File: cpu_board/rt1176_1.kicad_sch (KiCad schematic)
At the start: 46 parts, among them SW1 SWITCH_SMT4.6X2.8, U2 MIMXRT1176

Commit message: add models and power diagram
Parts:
- U2, U? (x4): footprint adcs:BGA289C80P17X17_1400X14000X152 -> adcs:U_MIMXRT1176DVMAA_NXP
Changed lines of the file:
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@@
       (effects (font (size 1.27 1.27)))
     )
-    (property "Footprint" "adcs:BGA289C80P17X17_1400X14000X152" (at 223.52 67.31 0)
+    (property "Footprint" "adcs:U_MIMXRT1176DVMAA_NXP" (at 223.52 67.31 0)
       (effects (font (size 1.27 1.27)) hide)
     )
@@
       (effects (font (size 1.27 1.27)) hide)
     )
+    (property "DigiKey Part Number" "" (at 223.52 66.04 0)
+      (effects (font (size 1.27 1.27)) hide)
+    )
+    (property "Tolerance" "" (at 223.52 66.04 0)
+      (effects (font (size 1.27 1.27)))
+    )
+    (property "Power Rating" "" (at 223.52 66.04 0)
+      (effects (font (size 1.27 1.27)))
+    )
     (pin "L9")
     (pin "M10")
@@
       (effects (font (size 1.27 1.27)))
     )
-    (property "Footprint" "adcs:BGA289C80P17X17_1400X14000X152" (at 220.98 142.24 0)
+    (property "Footprint" "adcs:U_MIMXRT1176DVMAA_NXP" (at 220.98 142.24 0)
       (effects (font (size 1.27 1.27)) hide)
     )
@@
       (effects (font (size 1.27 1.27)) hide)
     )
+    (property "DigiKey Part Number" "" (at 220.98 140.97 0)
+      (effects (font (size 1.27 1.27)) hide)
+    )
+    (property "Tolerance" "" (at 220.98 140.97 0)
+      (effects (font (size 1.27 1.27)))
+    )
+    (property "Power Rating" "" (at 220.98 140.97 0)
+      (effects (font (size 1.27 1.27)))
+    )
     (pin "L9")
     (pin "M10")
@@
       (effects (font (size 1.27 1.27)))
     )
-    (property "Footprint" "adcs:BGA289C80P17X17_1400X14000X152" (at 50.8 240.03 0)
+    (property "Footprint" "adcs:U_MIMXRT1176DVMAA_NXP" (at 50.8 240.03 0)
       (effects (font (size 1.27 1.27)) hide)
     )
@@
       (effects (font (size 1.27 1.27)) hide)
     )
+    (property "DigiKey Part Number" "" (at 50.8 238.76 0)
+      (effects (font (size 1.27 1.27)) hide)
+    )
+    (property "Tolerance" "" (at 50.8 238.76 0)
+      (effects (font (size 1.27 1.27)))
+    )
+    (property "Power Rating" "" (at 50.8 238.76 0)
+      (effects (font (size 1.27 1.27)))
+    )
     (pin "L9")
     (pin "M10")
@@
       (effects (font (size 1.27 1.27)))
     )
-    (property "Footprint" "adcs:BGA289C80P17X17_1400X14000X152" (at 220.98 200.66 0)
+    (property "Footprint" "adcs:U_MIMXRT1176DVMAA_NXP" (at 220.98 200.66 0)
       (effects (font (size 1.27 1.27)) hide)
     )
@@
       (effects (font (size 1.27 1.27)) hide)
     )
+    (property "DigiKey Part Number" "" (at 220.98 199.39 0)
+      (effects (font (size 1.27 1.27)) hide)
+    )
+    (property "Tolerance" "" (at 220.98 199.39 0)
+      (effects (font (size 1.27 1.27)))
+    )
+    (property "Power Rating" "" (at 220.98 199.39 0)
+      (effects (font (size 1.27 1.27)))
+    )
     (pin "L9")
     (pin "M10")
@@
       (effects (font (size 1.27 1.27)))
     )
-    (property "Footprint" "adcs:BGA289C80P17X17_1400X14000X152" (at 219.71 255.27 0)
+    (property "Footprint" "adcs:U_MIMXRT1176DVMAA_NXP" (at 219.71 255.27 0)
       (effects (font (size 1.27 1.27)) hide)
     )
@@
       (effects (font (size 1.27 1.27)) hide)
     )
+    (property "DigiKey Part Number" "" (at 219.71 254 0)
+      (effects (font (size 1.27 1.27)) hide)
+    )
+    (property "Tolerance" "" (at 219.71 254 0)
+      (effects (font (size 1.27 1.27)))
+    )
+    (property "Power Rating" "" (at 219.71 254 0)
+      (effects (font (size 1.27 1.27)))
+    )
     (pin "L9")

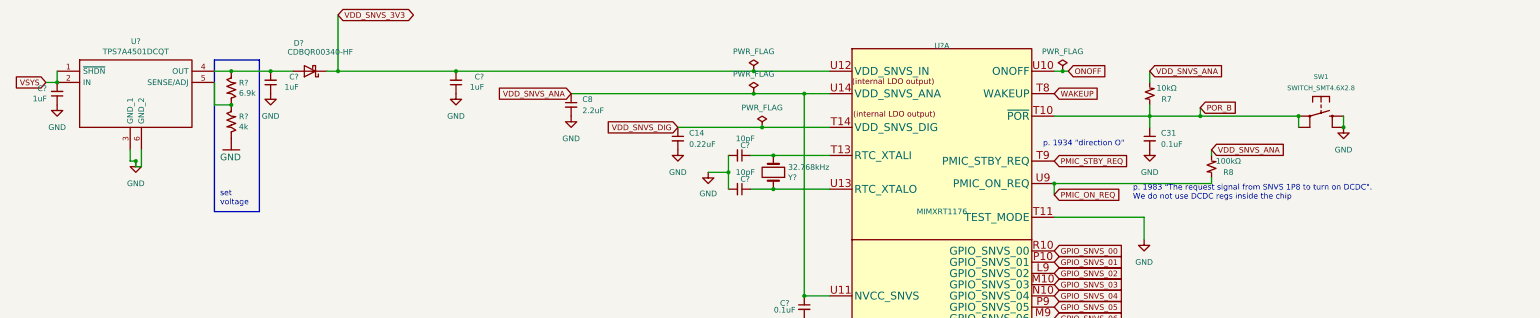
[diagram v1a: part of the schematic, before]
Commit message: continue work on fanout
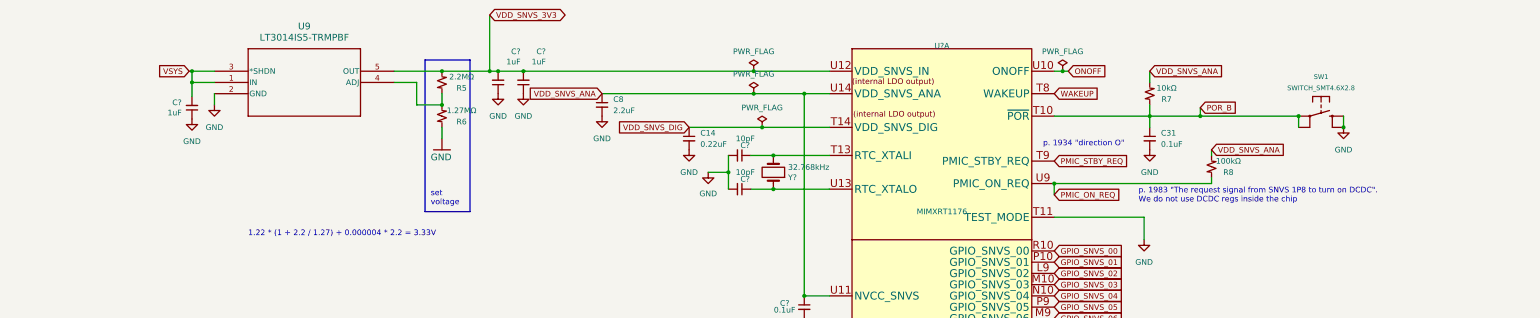
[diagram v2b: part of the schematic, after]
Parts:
- removed C?: 1uF, Capacitor_SMD:C_0402_1005Metric, symbol Device:C_Small
- removed D?: CDBQR00340-HF, adcs:D0402_H0.55MM, symbol Device:D_Schottky
- removed R?: 4k, Resistor_SMD:R_0402_1005Metric, symbol Device:R_US
- removed R?: 6.9k, Resistor_SMD:R_0402_1005Metric, symbol Device:R_US
- removed U?: TPS7A4501DCQT, mainboard:TPS7A4501DCQT, symbol mainboard:TPS7A4501DCQT
- added C?: 1uF, adcs:Perfect_0201, symbol Device:C_Small
- added R5: 2.2MΩ, adcs:Perfect_0402, symbol Device:R_Small_US
- added R6: 1.27MΩ, adcs:Perfect_0402, symbol Device:R_Small_US
- added U9: LT3014IS5-TRMPBF, adcs:S_5_ADI, symbol adcs:LT3014IS5-TRMPBF
- C10, C12, C13, C14, C15, C23, C26, C31, C34, C38, C40, C41, C42, C43, C8, C? (x3): footprint Capacitor_SMD:C_0402_1005Metric -> adcs:Perfect_0201
- C17, C22, C9: footprint Capacitor_SMD:C_0402_1005Metric -> adcs:Perfect_0201; Footprint (for JLCPCB) 0402 -> 0201
- C4, C? (x4): footprint Capacitor_SMD:C_0402_1005Metric -> adcs:Perfect_0402
- C6: footprint Capacitor_SMD:C_0402_1005Metric -> adcs:Perfect_0201; Footprint (for JLCPCB) 0402 -> 0201; Voltage Rating (none) -> 6.3V
- FB1, FB2: footprint Inductor_SMD:L_0402_1005Metric -> adcs:Perfect_0402
- R7, R8: footprint Resistor_SMD:R_0402_1005Metric -> adcs:Perfect_0402
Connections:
- net GND: now also C?.1, R6.1, U9.2 (GND)
- net VDD_SNVS_3V3: now also C?.2, R5.2, U9.5 (OUT)
- net VSYS: now also U9.1 (IN), U9.3 (*SHDN)
- new net: R5.1, R6.2, U9.4 (ADJ)
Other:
- note added: "1.22 * (1 + 2.2 / 1.27) + 0.000004 * 2.2 = 3.33V"
- moved on the sheet: C14, C8, C?

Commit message: grounded
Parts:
- C31, C? (x2): footprint adcs:Perfect_0201 -> adcs:Perfect_0402
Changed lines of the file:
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@@
       (effects (font (size 1.27 1.27)) (justify left))
     )
-    (property "Footprint" "adcs:Perfect_0201" (at 270.51 50.8 0)
+    (property "Footprint" "adcs:Perfect_0402" (at 270.51 50.8 0)
       (effects (font (size 1.27 1.27)) hide)
     )
@@
     (property "Footprint (for JLCPCB)" "0402" (at 270.51 50.8 0)
       (effects (font (size 1.27 1.27)) hide)
+    )
+    (property "DigiKey Part Number" "" (at 270.51 50.8 0)
+      (effects (font (size 1.27 1.27)) hide)
+    )
+    (property "Tolerance" "" (at 270.51 50.8 0)
+      (effects (font (size 1.27 1.27)))
+    )
+    (property "Power Rating" "" (at 270.51 50.8 0)
+      (effects (font (size 1.27 1.27)))
     )
     (pin "1")
@@
       (effects (font (size 1.27 1.27)) (justify left))
     )
-    (property "Footprint" "adcs:Perfect_0201" (at 53.975 43.815 0)
+    (property "Footprint" "adcs:Perfect_0402" (at 53.975 43.815 0)
       (effects (font (size 1.27 1.27)) hide)
     )
@@
     (property "Footprint (for JLCPCB)" "0402" (at 53.975 43.815 0)
       (effects (font (size 1.27 1.27)) hide)
+    )
+    (property "DigiKey Part Number" "" (at 53.975 43.815 0)
+      (effects (font (size 1.27 1.27)) hide)
+    )
+    (property "Tolerance" "" (at 53.975 43.815 0)
+      (effects (font (size 1.27 1.27)))
+    )
+    (property "Power Rating" "" (at 53.975 43.815 0)
+      (effects (font (size 1.27 1.27)))
     )
     (pin "1")
@@
       (effects (font (size 1.27 1.27)) (justify left))
     )
-    (property "Footprint" "adcs:Perfect_0201" (at 123.19 38.1 0)
-      (effects (font (size 1.27 1.27)) hide)
-    )
+    (property "Footprint" "adcs:Perfect_0402" (at 123.19 38.1 0)
+      (effects (font (size 1.27 1.27)) hide)
+    )
